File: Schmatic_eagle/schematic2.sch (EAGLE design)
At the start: 8 parts, among them IC1 MEGA16-A, IC2 MC145027DW, M1 WIRELESS-XY-MK-5V

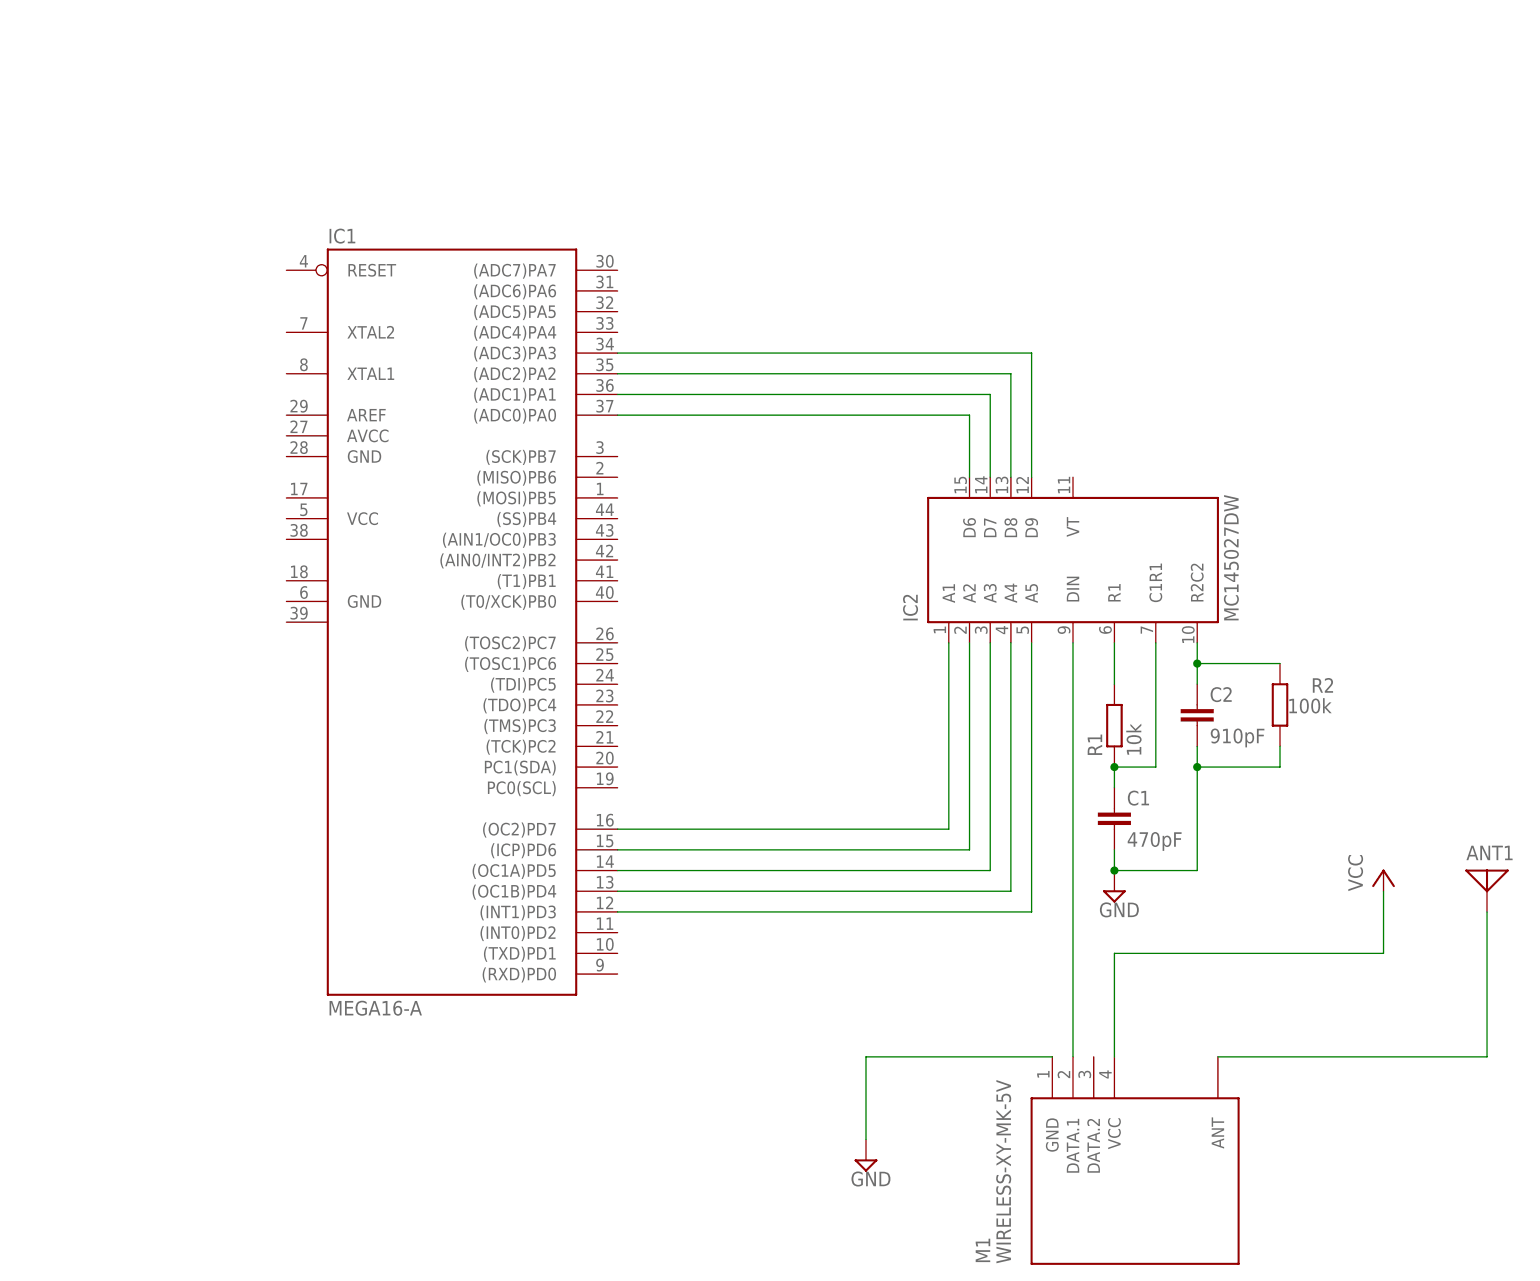
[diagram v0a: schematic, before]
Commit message: Schematic 2 updates
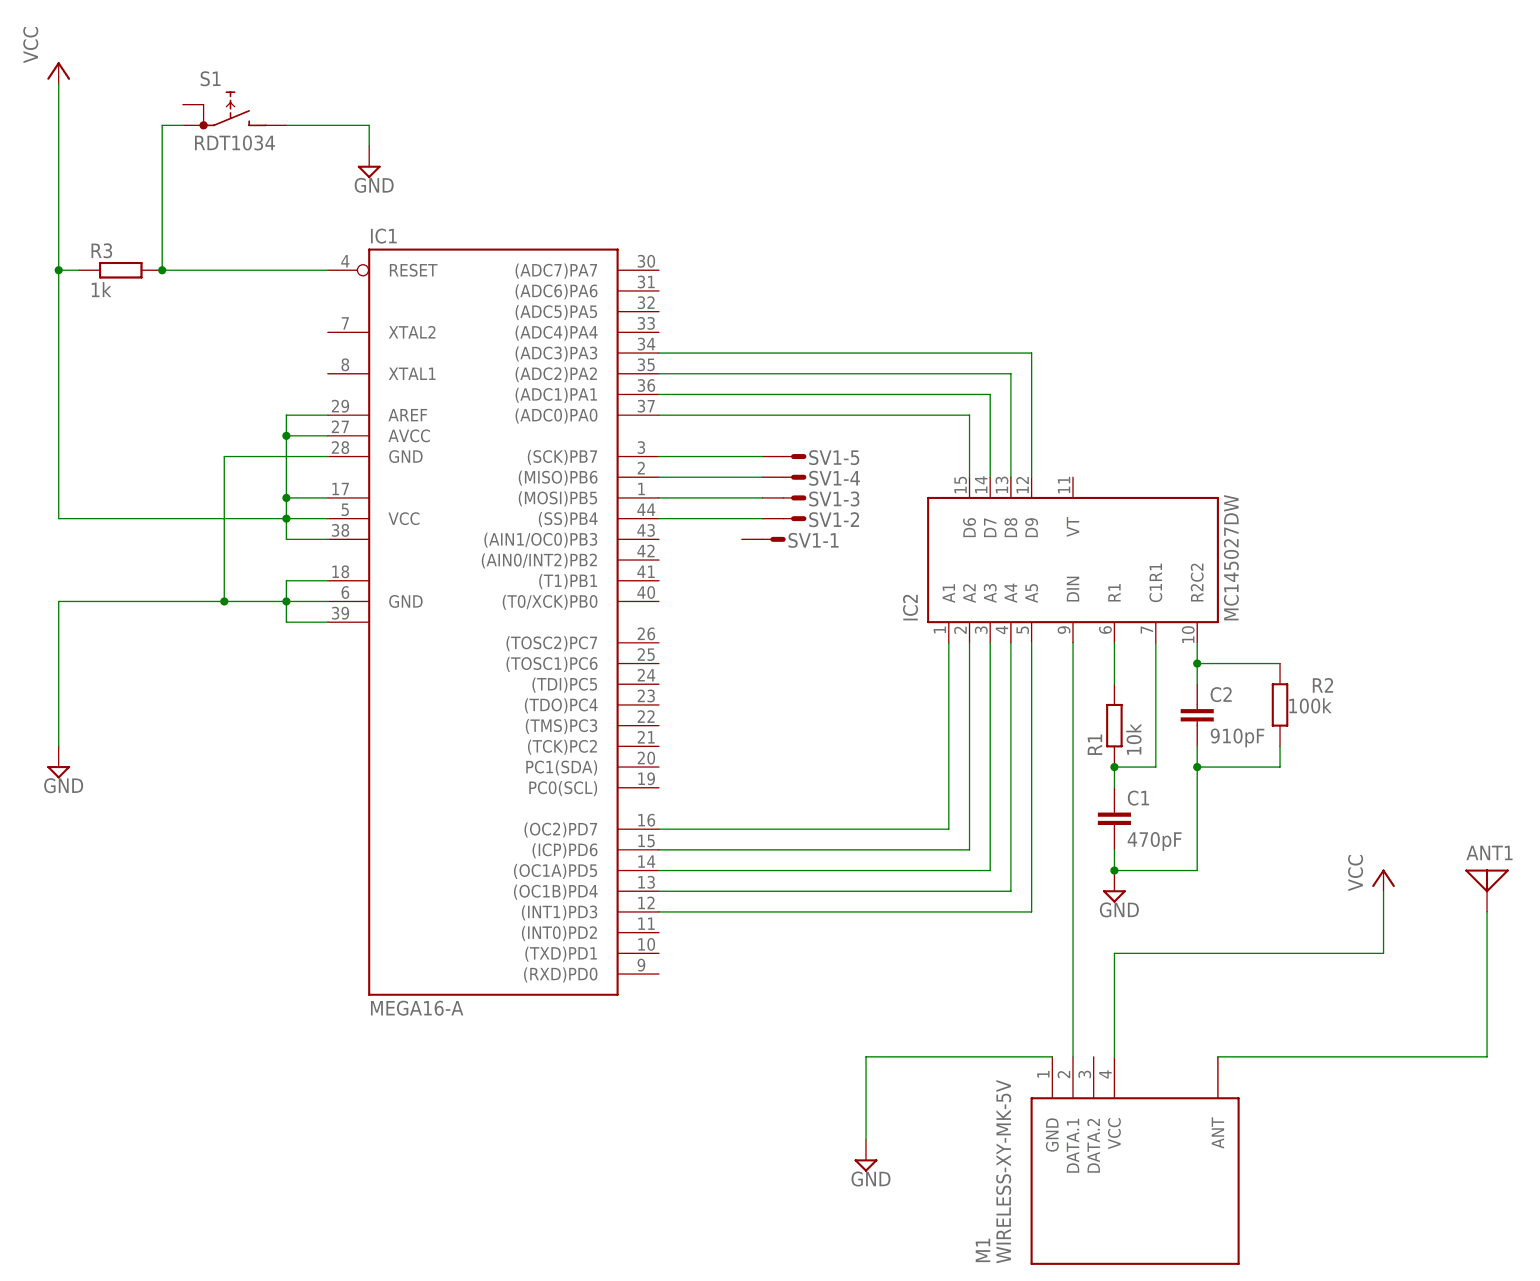
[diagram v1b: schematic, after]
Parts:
- added R3: 1k, rcl:R-EU_M0805
- added S1: RDT1034, switch:RDT1034
- added SV1: (no value), con-amp-mt:L05P
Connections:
- new net N$14: IC1.(SCK)PB7, SV1-5.S
- new net N$16: IC1.(MISO)PB6, SV1-4.S
- new net N$17: IC1.(MOSI)PB5, SV1-3.S
- new net N$18: IC1.(SS)PB4, SV1-2.S
- new net N$19: IC1.RESET, R3.2, S1.A1
- net GND: now also IC1.GND, IC1.GND1, IC1.GND2, IC1.GND@1, S1.B
- net VCC: now also IC1.AREF, IC1.AVCC, IC1.VCC, IC1.VCC1, IC1.VCC2, R3.1
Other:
- moved on the sheet: IC1
